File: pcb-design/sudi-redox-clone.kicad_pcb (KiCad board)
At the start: 2 copper layers, 123.4 x 99.4 mm, 127 parts, among them J1 SIDE_CON, J2 0.91 OLED, J3 SWD_JLINK, J5 SIDE_CON, J8 BatCon, K1 KEYSW, K10 KEYSW, K11 KEYSW, K12 KEYSW, K13 KEYSW, K14 KEYSW, K15 KEYSW, K16 KEYSW, K17 KEYSW, K18 KEYSW, K2 KEYSW, K3 KEYSW, K4 KEYSW, K5 KEYSW, K6 KEYSW, K7 KEYSW, K8 KEYSW, K9 KEYSW, P1 USB_C_Plug_USB2.0, SW1 RST, U4 AMS1117-3.3, U5 CH340C, U6 TP4056, U7 nRF52832-QFxx, U8 MCP23017_SS, Y5 32MHz

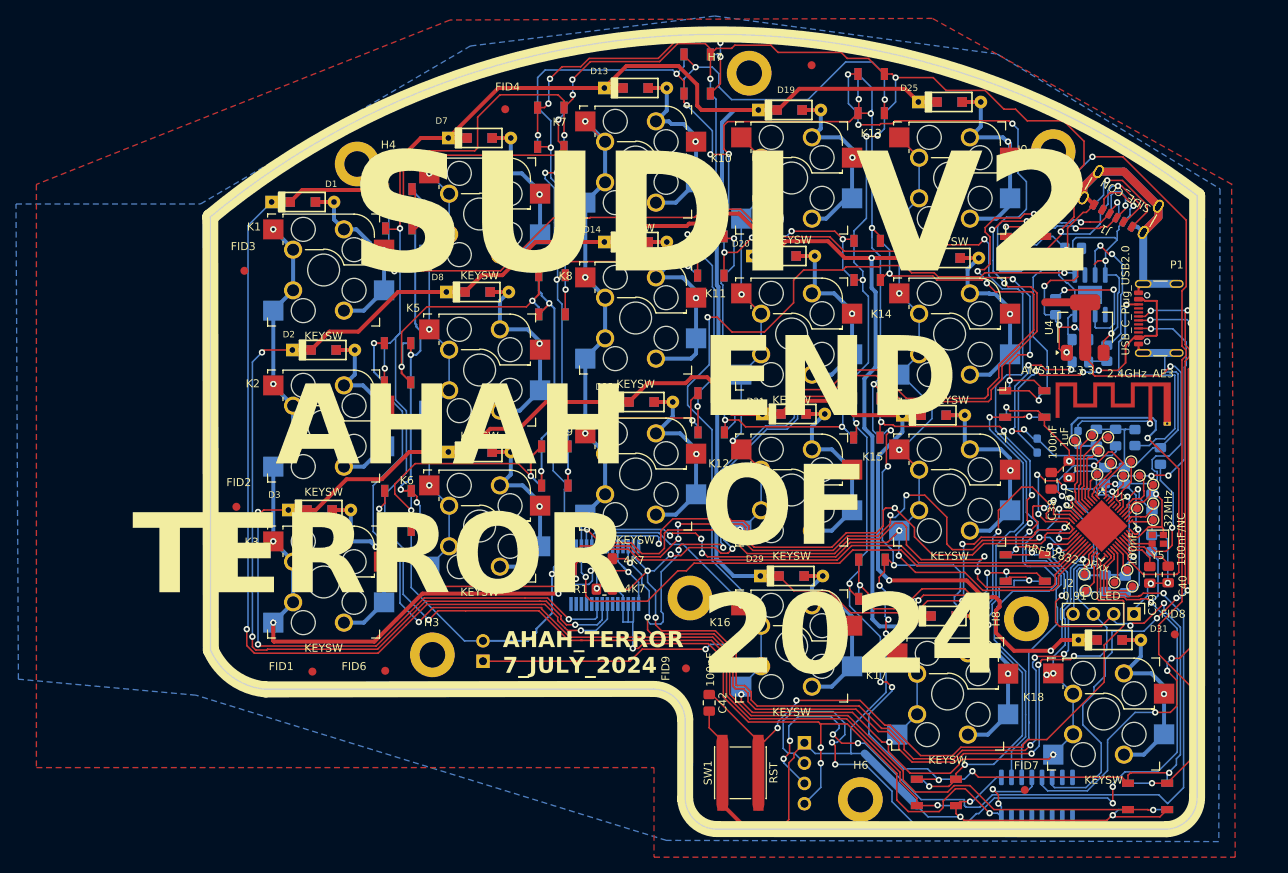
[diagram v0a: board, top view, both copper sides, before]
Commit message: [16-11-1807] change chargin mechanism
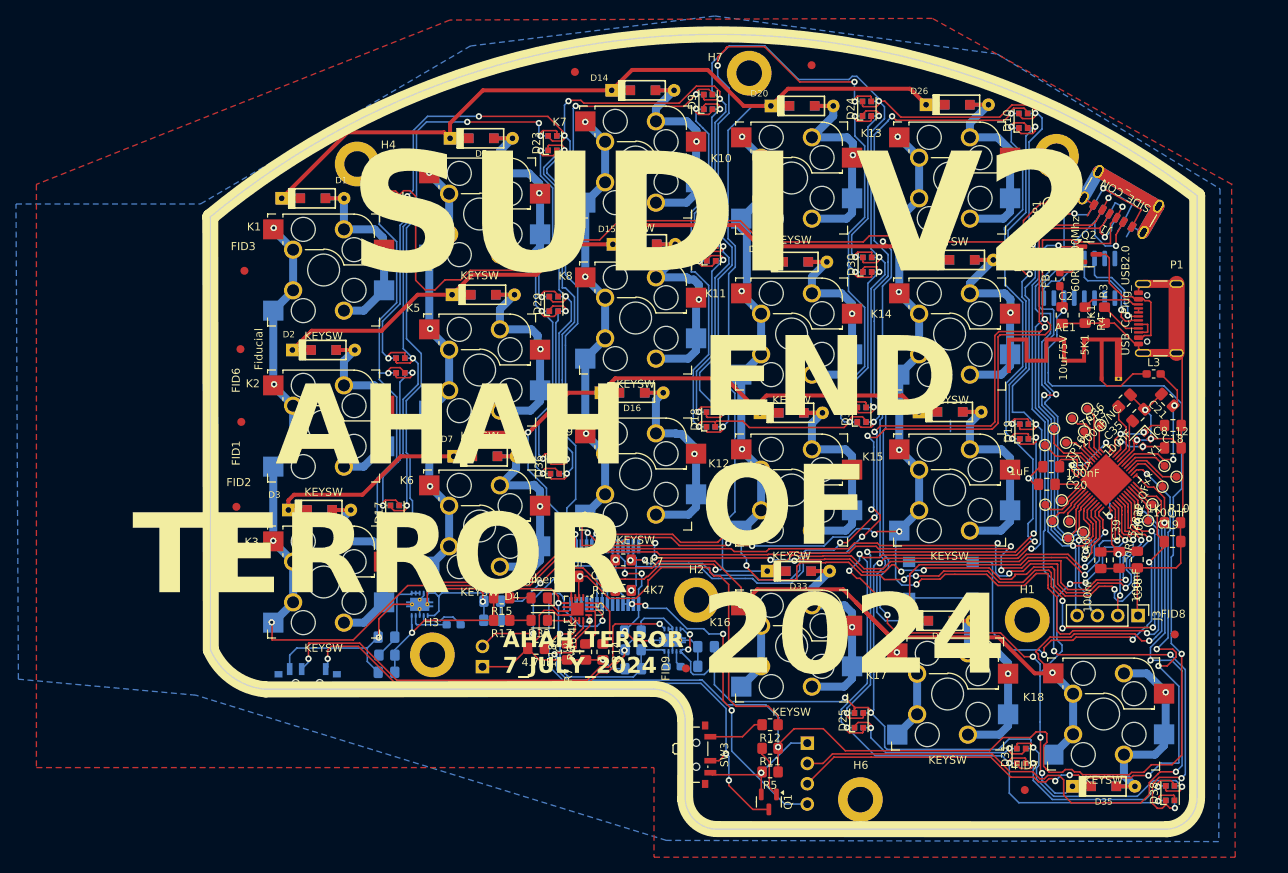
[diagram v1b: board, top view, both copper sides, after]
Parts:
- removed AE3: 2.4GHz, RF_Antenna:Texas_SWRA117D_2.4GHz_Left
- removed C41: 0.8pF, Capacitor_SMD:C_0805_2012Metric_Pad1.18x1.45mm_HandSolder
- removed C42: 100nF, Capacitor_SMD:C_0805_2012Metric_Pad1.18x1.45mm_HandSolder
- removed D43, D44, D45, D46, D47, D48: WS2812B, CustomWS2185BFootPrint:LED_WS2812B_PLCC4_5.0x5.0mm_P3.2mm
- removed H8, H9: MountingHole_Pad, MountingHole:MountingHole_3.2mm_M3_DIN965_Pad
- removed J8: BatCon, Connector_PinHeader_2.54mm:PinHeader_1x02_P2.54mm_Horizontal
- removed L7: 3.9nH, Inductor_SMD:L_0603_1608Metric_Pad1.05x0.95mm_HandSolder
- removed TPe (x2): TestPoint, TestPoint:TestPoint_Pad_D1.0mm
- removed Y5: 32MHz, Crystal:Crystal_SMD_2016-4Pin_2.0x1.6mm
- added AE1: 2.4GHz, RF_Antenna:Texas_SWRA117D_2.4GHz_Left, F.Cu at (219.8, 88.7)
- added C11: 0.1uF, Capacitor_SMD:C_0805_2012Metric_Pad1.18x1.45mm_HandSolder, B.Cu at (161.3, 120.2)
- added C12: 10uF, Capacitor_SMD:C_0805_2012Metric_Pad1.18x1.45mm_HandSolder, B.Cu at (170.4, 122.2)
- added C13: 10uF, Capacitor_SMD:C_0805_2012Metric_Pad1.18x1.45mm_HandSolder, B.Cu at (170.4, 124.7)
- added C14: 10uF, Capacitor_SMD:C_0805_2012Metric_Pad1.18x1.45mm_HandSolder, B.Cu at (130.4, 125.4)
- added C15: 0.1uF, Capacitor_SMD:C_0805_2012Metric_Pad1.18x1.45mm_HandSolder, B.Cu at (130.4, 121.0)
- added C16: 10uF, Capacitor_SMD:C_0805_2012Metric_Pad1.18x1.45mm_HandSolder, B.Cu at (143.7, 116.5)
- added C17: 10uF, Capacitor_SMD:C_0805_2012Metric_Pad1.18x1.45mm_HandSolder, B.Cu at (143.7, 118.9)
- added C18: 12pF, Capacitor_SMD:C_0805_2012Metric_Pad1.18x1.45mm_HandSolder, F.Cu at (228.8, 94.5)
- added C21: 0.8pF, Capacitor_SMD:C_0805_2012Metric_Pad1.18x1.45mm_HandSolder, F.Cu at (228.1, 91.3)
- added D32: red, LED_SMD:LED_0805_2012Metric_Pad1.15x1.40mm_HandSolder, F.Cu at (149.6, 118.9)
- added D33: 1N4148, canadian_footprints:D_SOD123_axial-dual, F.Cu at (181.9, 112.8)
- added D34: 1N4148, canadian_footprints:D_SOD123_axial-dual, F.Cu at (199.8, 119.0)
- added D35: 1N4148, canadian_footprints:D_SOD123_axial-dual, F.Cu at (220.1, 139.7)
- added D36: WS2812B, LED_SMD:LED_WS2812B-2020_PLCC4_2.0x2.0mm, F.Cu at (151.5, 99.7)
- added D37: WS2812B, LED_SMD:LED_WS2812B-2020_PLCC4_2.0x2.0mm, F.Cu at (189.8, 93.2)
- added D38: WS2812B, LED_SMD:LED_WS2812B-2020_PLCC4_2.0x2.0mm, F.Cu at (228.4, 140.5)
- added H1: MountingHole_Pad, MountingHole:MountingHole_3.2mm_M3_DIN965_Pad, F.Cu at (210.6, 118.8)
- added H2: MountingHole_Pad, MountingHole:MountingHole_3.2mm_M3_DIN965_Pad, F.Cu at (169.2, 116.3)
- added J4: BatCon, Connector_PinHeader_2.54mm:PinHeader_1x02_P2.54mm_Horizontal, B.Cu at (142.4, 124.7)
- added JP1: END_TX, Jumper:SolderJumper-2_P1.3mm_Open_RoundedPad1.0x1.5mm, F.Cu at (213.6, 67.5)
- added L1: 22uH, Inductor_SMD:L_0603_1608Metric_Pad1.05x0.95mm_HandSolder, B.Cu at (166.3, 124.7)
- added L2: 22uH, Inductor_SMD:L_0603_1608Metric_Pad1.05x0.95mm_HandSolder, B.Cu at (138.8, 119.5)
- added L3: 3.9nH, Inductor_SMD:L_0603_1608Metric_Pad1.05x0.95mm_HandSolder, F.Cu at (226.3, 88.1)
- added Q1: PJA3404_(G1,D3,S2), Package_TO_SOT_SMD:SOT-23, F.Cu at (178.2, 141.6)
- added Q2: PJA3405_(G1,D3,S2), Package_TO_SOT_SMD:SOT-23, F.Cu at (218.2, 73.2)
- added R11: 1k, Resistor_SMD:R_0805_2012Metric_Pad1.20x1.40mm_HandSolder, F.Cu at (178.4, 134.9)
- added R12: 100k, Resistor_SMD:R_0805_2012Metric_Pad1.20x1.40mm_HandSolder, F.Cu at (178.4, 131.9)
- added R13: 100, Resistor_SMD:R_0805_2012Metric_Pad1.20x1.40mm_HandSolder, B.Cu at (161.3, 122.6)
- added R14: 1.13k, Resistor_SMD:R_0805_2012Metric_Pad1.20x1.40mm_HandSolder, F.Cu at (157.5, 122.8)
- added R15: 1K, Resistor_SMD:R_0805_2012Metric_Pad1.20x1.40mm_HandSolder, F.Cu at (144.8, 116.1)
- added R16: 100, Resistor_SMD:R_0805_2012Metric_Pad1.20x1.40mm_HandSolder, B.Cu at (130.5, 123.2)
- added R17: 1K, Resistor_SMD:R_0805_2012Metric_Pad1.20x1.40mm_HandSolder, F.Cu at (144.8, 118.9)
- added R5: 100k, Resistor_SMD:R_0805_2012Metric_Pad1.20x1.40mm_HandSolder, F.Cu at (178.4, 137.8)
- added SW3: PWR_SWITCH, Button_Switch_SMD:SW_SPDT_PCM12, F.Cu at (169.5, 135.7)
- added SW4: 5V_EN, Button_Switch_SMD:SW_SPDT_PCM12, B.Cu at (120.6, 126.4)
- added TP13: TestPoint, TestPoint:TestPoint_Pad_D1.0mm, F.Cu at (218.1, 92.5)
- added TP16: TestPoint, TestPoint:TestPoint_Pad_D1.0mm, F.Cu at (215.4, 96.7)
- added U9: TPS63001_SEPIC_3V3, Package_SON:Texas_DRC0010J_ThermalVias, B.Cu at (134.6, 116.9)
- added Y1: 32MHz_CF4032M00020001, Crystal:Crystal_SMD_2016-4Pin_2.0x1.6mm, F.Cu at (225.1, 96.3)
- C1: value 10uF -> 4.7uF; moved to F.Cu
- C19: value 12pF -> 100nF; moved to F.Cu
- C2, C20, C35, C8, FB1, R10, R3, R4: moved to F.Cu
- C3: value 10uF/5V -> 4.7uF; moved to F.Cu
- C36: value 100nF -> 100nF/NC; moved to F.Cu
- C40: value 100nF/NC -> 100nF
- D1, D14, D15, D2, D20, D21, D26, D27, D3, D7: value 1N5820 -> 1N4148
- D10, D12, D17, D18, D23, D24: footprint CustomWS2185BFootPrint:LED_WS2812B_PLCC4_5.0x5.0mm_P3.2mm -> LED_SMD:LED_WS2812B-2020_PLCC4_2.0x2.0mm; moved to F.Cu
- D11: footprint CustomWS2185BFootPrint:LED_WS2812B_PLCC4_5.0x5.0mm_P3.2mm -> LED_SMD:LED_WS2812B-2020_PLCC4_2.0x2.0mm
- D13, D19, D25, D29, D30, D31, D8, D9: value 1N5820 -> WS2812B; footprint canadian_footprints:D_SOD123_axial-dual -> LED_SMD:LED_WS2812B-2020_PLCC4_2.0x2.0mm
- D16, D5: value WS2812B -> 1N4148; footprint CustomWS2185BFootPrint:LED_WS2812B_PLCC4_5.0x5.0mm_P3.2mm -> canadian_footprints:D_SOD123_axial-dual; moved to F.Cu
- D22, D28, D6: value WS2812B -> 1N4148; footprint CustomWS2185BFootPrint:LED_WS2812B_PLCC4_5.0x5.0mm_P3.2mm -> canadian_footprints:D_SOD123_axial-dual
- D4: value RED -> green; moved to F.Cu
- J2: value 0.91 OLED -> SWD_JLINK; footprint Connector_PinHeader_2.54mm:PinHeader_1x04_P2.54mm_Vertical -> Connector_PinHeader_2.54mm:PinHeader_1x04_P2.54mm_Horizontal; moved to B.Cu
- J3: value SWD_JLINK -> 0.91 OLED; footprint Connector_PinHeader_2.54mm:PinHeader_1x04_P2.54mm_Horizontal -> Connector_PinHeader_2.54mm:PinHeader_1x04_P2.54mm_Vertical; moved to F.Cu
- R6: value 1K -> 46.4K; moved to F.Cu
- R7: value 1.2 -> 1.18k; moved to F.Cu
- SW1: moved to B.Cu
- U4: value AMS1117-3.3 -> CH340C; footprint Package_TO_SOT_SMD:SOT-223-3_TabPin2 -> Package_SO:SOIC-16_3.9x9.9mm_P1.27mm; moved to B.Cu
- U5: value CH340C -> BQ24075RGT_DPPM; footprint Package_SO:SOIC-16_3.9x9.9mm_P1.27mm -> Package_DFN_QFN:VQFN-16-1EP_3x3mm_P0.5mm_EP1.6x1.6mm; moved to F.Cu
- U6: value TP4056 -> TPS63002_SEPIC_5V; footprint Package_SO:SOIC-8-1EP_3.9x4.9mm_P1.27mm_EP2.29x3mm -> Package_SON:Texas_DRC0010J_ThermalVias
- moved D25 78.1 mm to (189.5, 131.4), turned to 90 degrees
- moved C3 76.6 mm to (149.2, 122.4), turned to 180 degrees
- moved C4 76.1 mm to (161.3, 125.0)
- moved R6 75.1 mm to (155.3, 122.8)
- moved R7 74.7 mm to (153.1, 122.8), turned to -90 degrees
- moved D4 73.8 mm to (149.5, 116.1)
- moved C1 70.3 mm to (153.4, 113.4), turned to 180 degrees
- moved U6 67.7 mm to (166.2, 121.4)
- moved D16 62.8 mm to (161.2, 90.5), turned to 0 degrees
- moved U5 62.1 mm to (154.3, 117.5)
- moved D24 60.7 mm to (190.5, 55.0), turned to 90 degrees
- moved D11 59.8 mm to (132.2, 87.0), turned to 90 degrees
- moved D13 53.1 mm to (210.2, 73.8), turned to 90 degrees
- moved D9 52.3 mm to (170.7, 54.1), turned to 90 degrees
- moved D23 52.2 mm to (151.2, 59.2), turned to 90 degrees
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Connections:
- net Tx renamed END_TX
- C1 pad 1: +5V -> +BATT
- C19 pad 1: GND -> Net-(U7-P0.21/~{RESET})
- C19 pad 2: Net-(U7-XC2) -> GND
- C2 pad 1: +5V -> VBUS
- C20 pad 1: +3.3V -> GND
- C20 pad 2: GND -> Net-(U7-DEC1)
- C3 pad 1: +3.3V -> VDD
- C35 pad 1: +3.3V -> GND
- C35 pad 2: GND -> Net-(U7-DEC2)
- C36 pad 1: +3.3V -> GND
- C36 pad 2: GND -> Net-(U7-DEC3)
- C38 pad 1: GND -> +3.3V
- C38 pad 2: Net-(U7-DEC1) -> GND
- C39 pad 1: GND -> +3.3V
- C39 pad 2: Net-(U7-DEC2) -> GND
- C4 pad 1: Net-(J8-Pin_1) -> VDD
- C40 pad 1: GND -> +3.3V
- C40 pad 2: Net-(U7-DEC3) -> GND
- D10 pad 1: +3V7 -> Net-(D10-DOUT)
- D10 pad 2: Net-(D10-DOUT) -> GND
- D10 pad 3: GND -> /DOUT2
- D10 pad 4: Net-(D10-DIN) -> +5V
- D11 pad 1: +3V7 -> Net-(D11-DOUT)
- D11 pad 2: Net-(D11-DOUT) -> GND
- D11 pad 3: GND -> Net-(D11-DIN)
- D11 pad 4: Net-(D10-DOUT) -> +5V
- D12 pad 1: +3V7 -> Net-(D12-DOUT)
- D12 pad 2: Net-(D12-DOUT) -> GND
- D12 pad 3: GND -> Net-(D12-DIN)
- D12 pad 4: Net-(D11-DOUT) -> +5V
- D13 pad 1: row1 -> Net-(D13-DOUT)
- D13 pad 2: Net-(D13-A) -> GND
- D14 pad 1: row2 -> row1
- D15 pad 1: row3 -> row2
- D16 pad 1: +3V7 -> row3
- D16 pad 2: Net-(D16-DOUT) -> Net-(D16-A)
- D17 pad 1: +3V7 -> Net-(D17-DOUT)
- D17 pad 2: Net-(D17-DOUT) -> GND
- D17 pad 3: GND -> Net-(D11-DOUT)
- D17 pad 4: Net-(D16-DOUT) -> +5V
- D18 pad 1: +3V7 -> Net-(D18-DOUT)
- D18 pad 2: Net-(D18-DOUT) -> GND
- D18 pad 3: GND -> Net-(D12-DOUT)
- D18 pad 4: Net-(D17-DOUT) -> +5V
- D19 pad 1: row1 -> Net-(D19-DOUT)
- D19 pad 2: Net-(D19-A) -> GND
- D20 pad 1: row2 -> row1
- D21 pad 1: row3 -> row2
- D22 pad 1: +3V7 -> row3
- D22 pad 2: Net-(D22-DOUT) -> Net-(D22-A)
- D23 pad 1: +3V7 -> Net-(D23-DOUT)
- D23 pad 2: Net-(D23-DOUT) -> GND
- D23 pad 3: GND -> Net-(D17-DOUT)
- D23 pad 4: Net-(D22-DOUT) -> +5V
- D24 pad 1: +3V7 -> Net-(D24-DOUT)
- D24 pad 2: Net-(D24-DOUT) -> GND
- D24 pad 3: GND -> Net-(D18-DOUT)
- D24 pad 4: Net-(D23-DOUT) -> +5V
- D25 pad 1: row1 -> Net-(D25-DOUT)
- D25 pad 2: Net-(D25-A) -> GND
- D26 pad 1: row2 -> row1
- D27 pad 1: row3 -> row2
- D28 pad 1: +3V7 -> row3
- D28 pad 2: unconnected-(D28-DOUT-Pad2) -> Net-(D28-A)
- D29 pad 1: row1 -> Net-(D29-DOUT)
- D29 pad 2: Net-(D29-A) -> GND
- D30 pad 1: row2 -> Net-(D30-DOUT)
- D30 pad 2: Net-(D30-A) -> GND
- D31 pad 1: row3 -> Net-(D31-DOUT)
- D31 pad 2: Net-(D31-A) -> GND
- D4 pad 2: +5V -> Net-(D4-A)
- D5 pad 1: +3V7 -> row1
- D5 pad 2: Net-(D5-DOUT) -> Net-(D5-A)
- D6 pad 1: +3V7 -> row2
- D6 pad 2: Net-(D10-DIN) -> Net-(D6-A)
- D7 pad 1: row1 -> row3
- D8 pad 1: row2 -> Net-(D11-DIN)
- D8 pad 2: Net-(D8-A) -> GND
- D9 pad 1: row3 -> Net-(D12-DIN)
- D9 pad 2: Net-(D9-A) -> GND
- FB1 pad 1: Net-(FB1-Pad1) -> Net-(Q2-S)
- FB1 pad 2: +5V -> VBUS
- J1 pad B9: +3V7 -> +3.3V
- J2 pad 2: +3V7 -> /SWCLK
- J2 pad 3: SCL -> /SWDIO
- J2 pad 4: SDA -> +3.3V
- J3 pad 2: /SWCLK -> +3.3V
- J3 pad 3: /SWDIO -> SCL
- J3 pad 4: +3.3V -> SDA
- J5 pad B9: +3V7 -> +3.3V
- K10 pad 2: Net-(D19-A) -> Net-(D20-A)
- K11 pad 2: Net-(D20-A) -> Net-(D21-A)
- K12 pad 2: Net-(D21-A) -> Net-(D22-A)
- K13 pad 2: Net-(D25-A) -> Net-(D26-A)
- K14 pad 2: Net-(D26-A) -> Net-(D27-A)
- K15 pad 2: Net-(D27-A) -> Net-(D28-A)
- K16 pad 2: Net-(D29-A) -> Net-(D33-A)
- K17 pad 2: Net-(D30-A) -> Net-(D34-A)
- K18 pad 2: Net-(D31-A) -> Net-(D35-A)
- K4 pad 2: Net-(D7-A) -> Net-(D5-A)
- K5 pad 2: Net-(D8-A) -> Net-(D6-A)
- K6 pad 2: Net-(D9-A) -> Net-(D7-A)
- K7 pad 2: Net-(D13-A) -> Net-(D14-A)
- K8 pad 2: Net-(D14-A) -> Net-(D15-A)
- K9 pad 2: Net-(D15-A) -> Net-(D16-A)
- P1 pad A4: Net-(FB1-Pad1) -> Net-(Q2-D)
- P1 pad A9: Net-(FB1-Pad1) -> Net-(Q2-D)
- P1 pad B4: Net-(FB1-Pad1) -> Net-(Q2-D)
- P1 pad B9: Net-(FB1-Pad1) -> Net-(Q2-D)
- R6 pad 1: Net-(U6-~{CHRG}) -> /TMR
- R6 pad 2: Net-(D4-K) -> GND
- R7 pad 1: GND -> /ILIM
- R7 pad 2: Net-(U6-PROG) -> GND
- TP1 pad 1: /P0.19 -> /P0.00/XL1
- TP10 pad 1: /P0.29/AIN5 -> /P0.23
- TP11 pad 1: /P0.30/AIN6 -> /P0.24
- TP12 pad 1: /P0.31/AIN7 -> /P0.25
- TP14 pad 1: /P0.01/XL2 -> /P0.27
- TP15 pad 1: /P0.02/AIN0 -> /P0.28/AIN4
- TP17 pad 1: /P0.04/AIN2 -> /P0.30/AIN6
- TP18 pad 1: /P0.05/AIN3 -> /P0.31/AIN7
- TP2 pad 1: /P0.22 -> /P0.01/XL2
- TP3 pad 1: /P0.20 -> /P0.02/AIN0
- TP4 pad 1: /P0.23 -> /P0.03/AIN1
- TP5 pad 1: /P0.24 -> /P0.04/AIN2
- TP6 pad 1: /P0.25 -> /P0.05/AIN3
- TP7 pad 1: /P0.26 -> /P0.19
- TP8 pad 1: /P0.27 -> /P0.20
- TP9 pad 1: /P0.28/AIN4 -> /P0.22
- U4 pad 2: +3.3V -> RX
- U4 pad 3: +5V -> TX
- U5 pad 1: GND -> unconnected-(U5-TS-Pad1)
- U5 pad 10: unconnected-(U5-~{DSR}-Pad10) -> VDD
- U5 pad 11: unconnected-(U5-~{RI}-Pad11) -> VDD
- U5 pad 12: unconnected-(U5-~{DCD}-Pad12) -> /ILIM
- U5 pad 13: unconnected-(U5-~{DTR}-Pad13) -> VBUS
- U5 pad 14: unconnected-(U5-~{RTS}-Pad14) -> /TMR
- U5 pad 15: unconnected-(U5-R232-Pad15) -> /SYSOFF
- U5 pad 16: +3.3V -> /ISET
- U5 pad 2: RX -> +BATT
- U5 pad 3: TX -> +BATT
- U5 pad 4: +3.3V -> GND
- U5 pad 5: Net-(P1-D+) -> VDD
- U5 pad 6: Net-(P1-D-) -> GND
- U5 pad 7: unconnected-(U5-NC-Pad7) -> Net-(D4-K)
- U5 pad 8: unconnected-(U5-~{OUT}/~{DTR}-Pad8) -> GND
- U5 pad 9: unconnected-(U5-~{CTS}-Pad9) -> Net-(D32-K)
- U6 pad 1: unconnected-(U6-TEMP-Pad1) -> +5V
- U6 pad 2: Net-(U6-PROG) -> Net-(U6-L2)
- U6 pad 4: +5V -> Net-(U6-L1)
- U6 pad 5: Net-(J8-Pin_1) -> VDD
- U6 pad 6: unconnected-(U6-~{STDBY}-Pad6) -> Net-(SW4-B)
- U6 pad 7: Net-(U6-~{CHRG}) -> Net-(SW4-A)
- U6 pad 8: +5V -> Net-(SW4-A)
- U6 pad 9: unconnected-(U6-PP-Pad9) -> GND
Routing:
- net +3V7: track 539.7 -> 0.00 mm, vias 32 -> 0
- net +5V: track 84.9 -> 558.7 mm, vias 7 -> 26
- net VBUS: track 0.00 -> 183.0 mm, vias 0 -> 5
- net Net-(D48-DOUT): track 150.7 -> 0.00 mm, vias 3 -> 0
- net +3.3V: track 278.5 -> 140.8 mm, vias 16 -> 13
- net Net-(J8-Pin_1): track 134.6 -> 0.00 mm, vias 3 -> 0
- net Net-(D47-DOUT): track 114.3 -> 0.00 mm, vias 4 -> 0
- net END_TX: track 13.5 -> 116.9 mm, vias 1 -> 7
- net Net-(D16-DOUT): track 99.9 -> 0.00 mm, vias 3 -> 0
- net row1: track 322.3 -> 231.4 mm
- net SCL: track 244.4 -> 156.3 mm, vias 14 -> 8
- net /DOUT1: track 0.00 -> 72.8 mm, vias 0 -> 3
- net Net-(P1-D-): track 81.8 -> 11.3 mm, vias 5 -> 1
- net Net-(P1-D+): track 82.4 -> 13.3 mm, vias 5 -> 1
- net +BATT: track 0.00 -> 67.2 mm, vias 0 -> 2
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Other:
- board text added: "FINISHED AT 16 NOV 2024"
- board text removed: "FINISHED AT 1 NOV 2024"
